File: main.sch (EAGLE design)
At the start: 34 parts, among them IC1 ATTINY13A-SSH, T1A 2N4401, T1B NPN, T2A 2N4401, T2B NPN

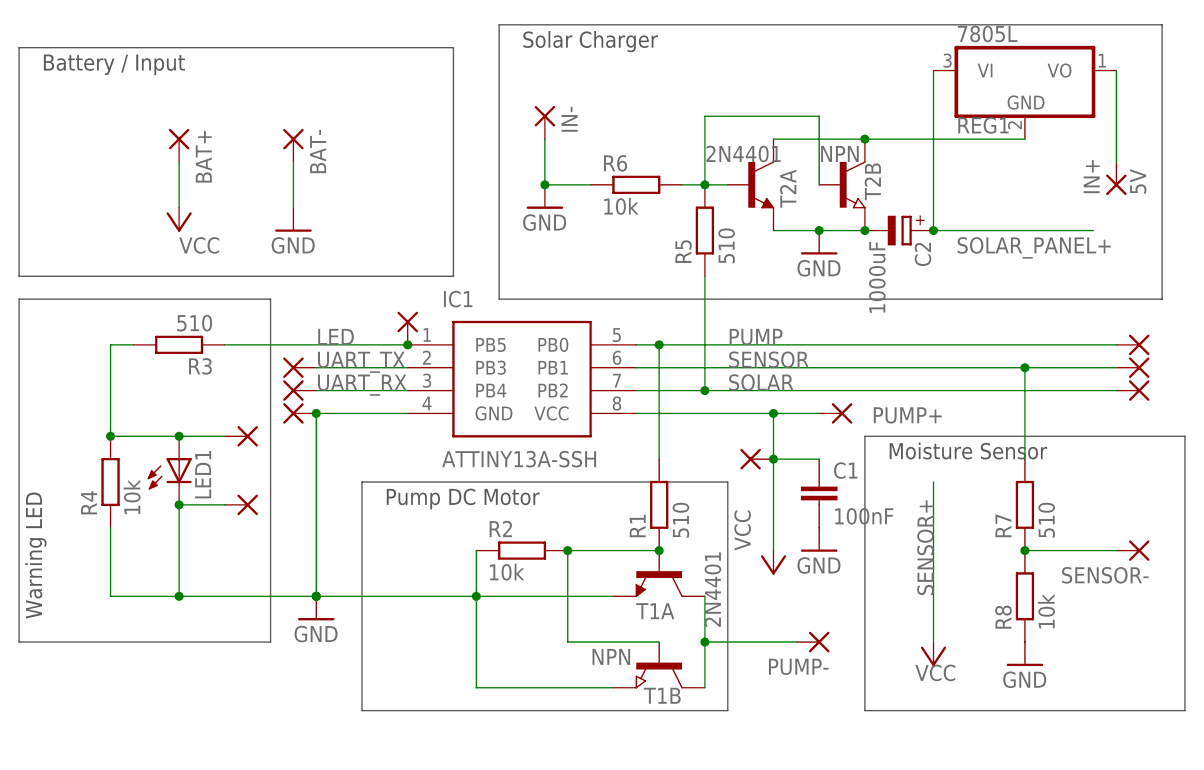
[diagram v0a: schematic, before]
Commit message: optimized pcb and code
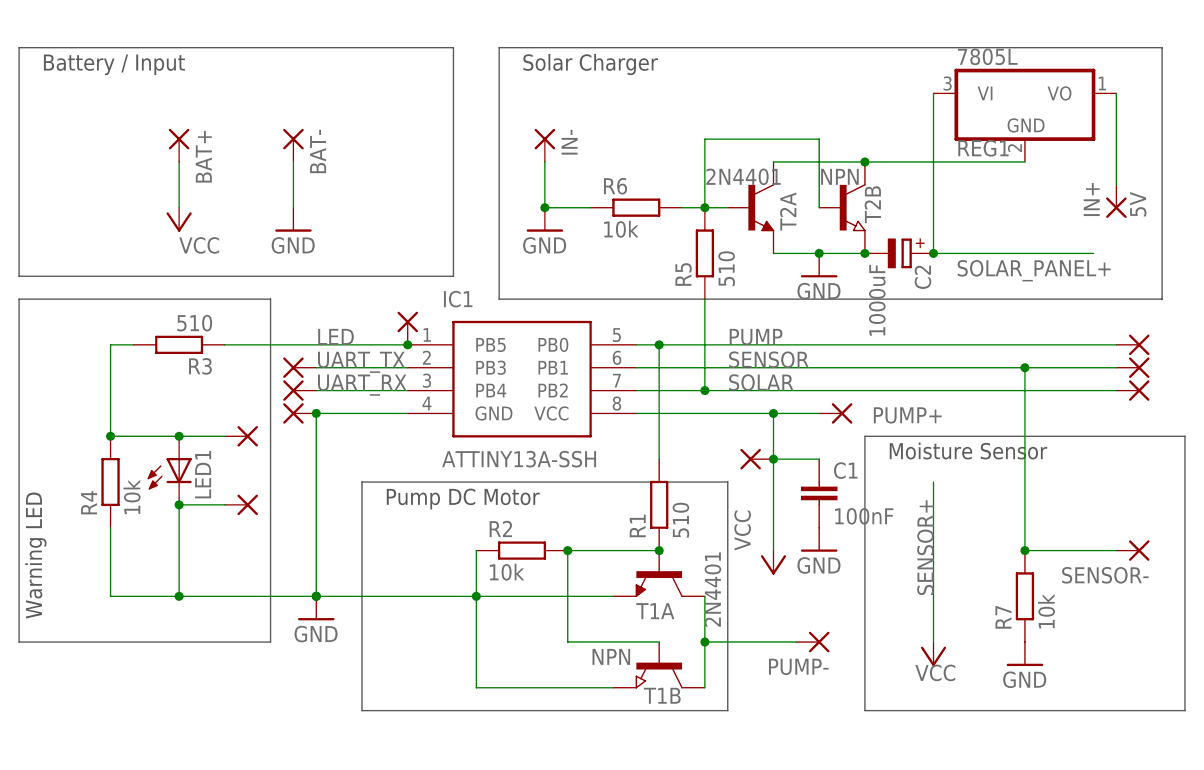
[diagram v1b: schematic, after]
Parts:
- removed R8: 10k, resistor:R-EU_M0805
- R7: value 510 -> 10k
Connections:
- removed net N$7: R7.1, R8.2, SENSOR-.P
- net GND: now also R7.1; no longer R8.1
- net SENSOR: now also SENSOR-.P
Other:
- moved on the sheet: C2, IN+, IN-, R5, R6, R7, REG1, T2A, T2B

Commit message: Rev 0.3
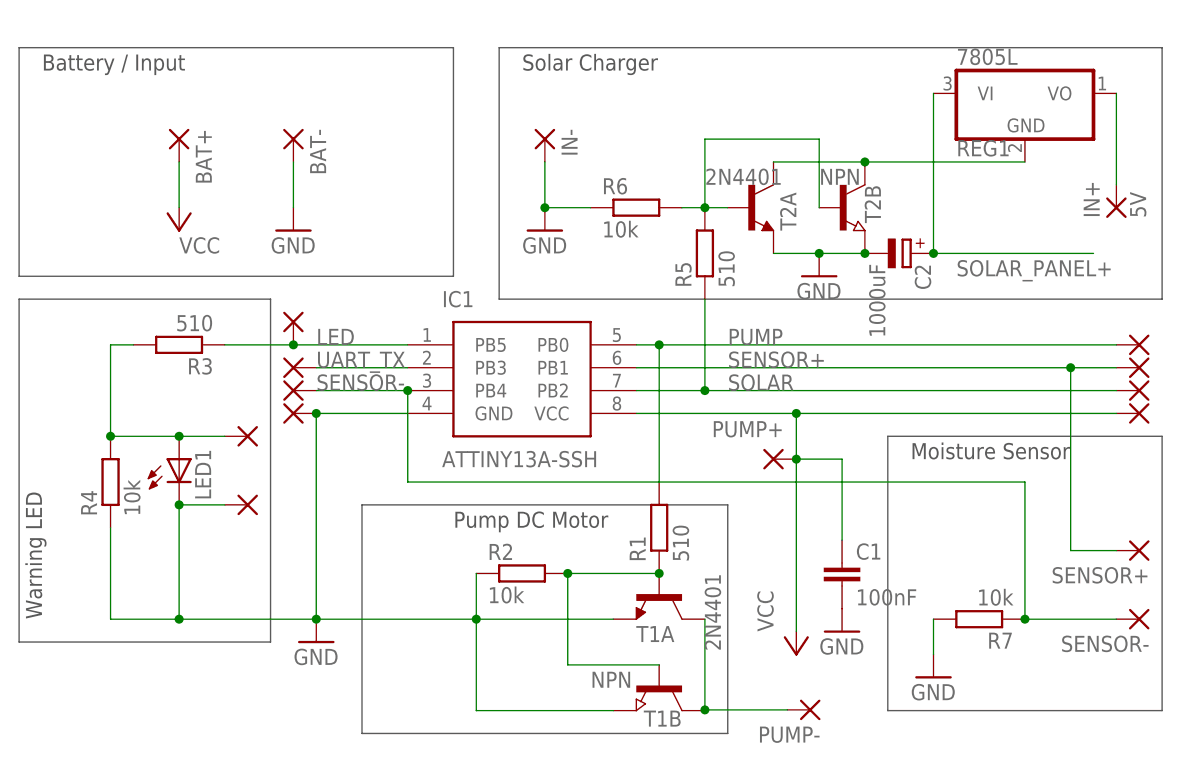
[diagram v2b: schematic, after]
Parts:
- added SENSOR+: (no value), wirepad:1,6/0,8
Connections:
- removed net SENSOR: IC1.PB1, PAD6.P, R7.2, SENSOR-.P
- removed net UART_RX: IC1.PB4, PAD8.P
- new net SENSOR+: IC1.PB1, PAD6.P, SENSOR+.P
- new net SENSOR-: IC1.PB4, PAD8.P, R7.1, SENSOR-.P
- net GND: now also R7.2; no longer R7.1
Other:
- moved on the sheet: C1, PUMP+, PUMP-, R1, R2, R7, SENSOR-, T1A, T1B
